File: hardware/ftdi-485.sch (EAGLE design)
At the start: 35 parts, among them IC1 MAX481CSA, J1 NE8FAH, J2 POWER_JACKPTH_LOCK, U1 FT232BL, Y1 6MHz

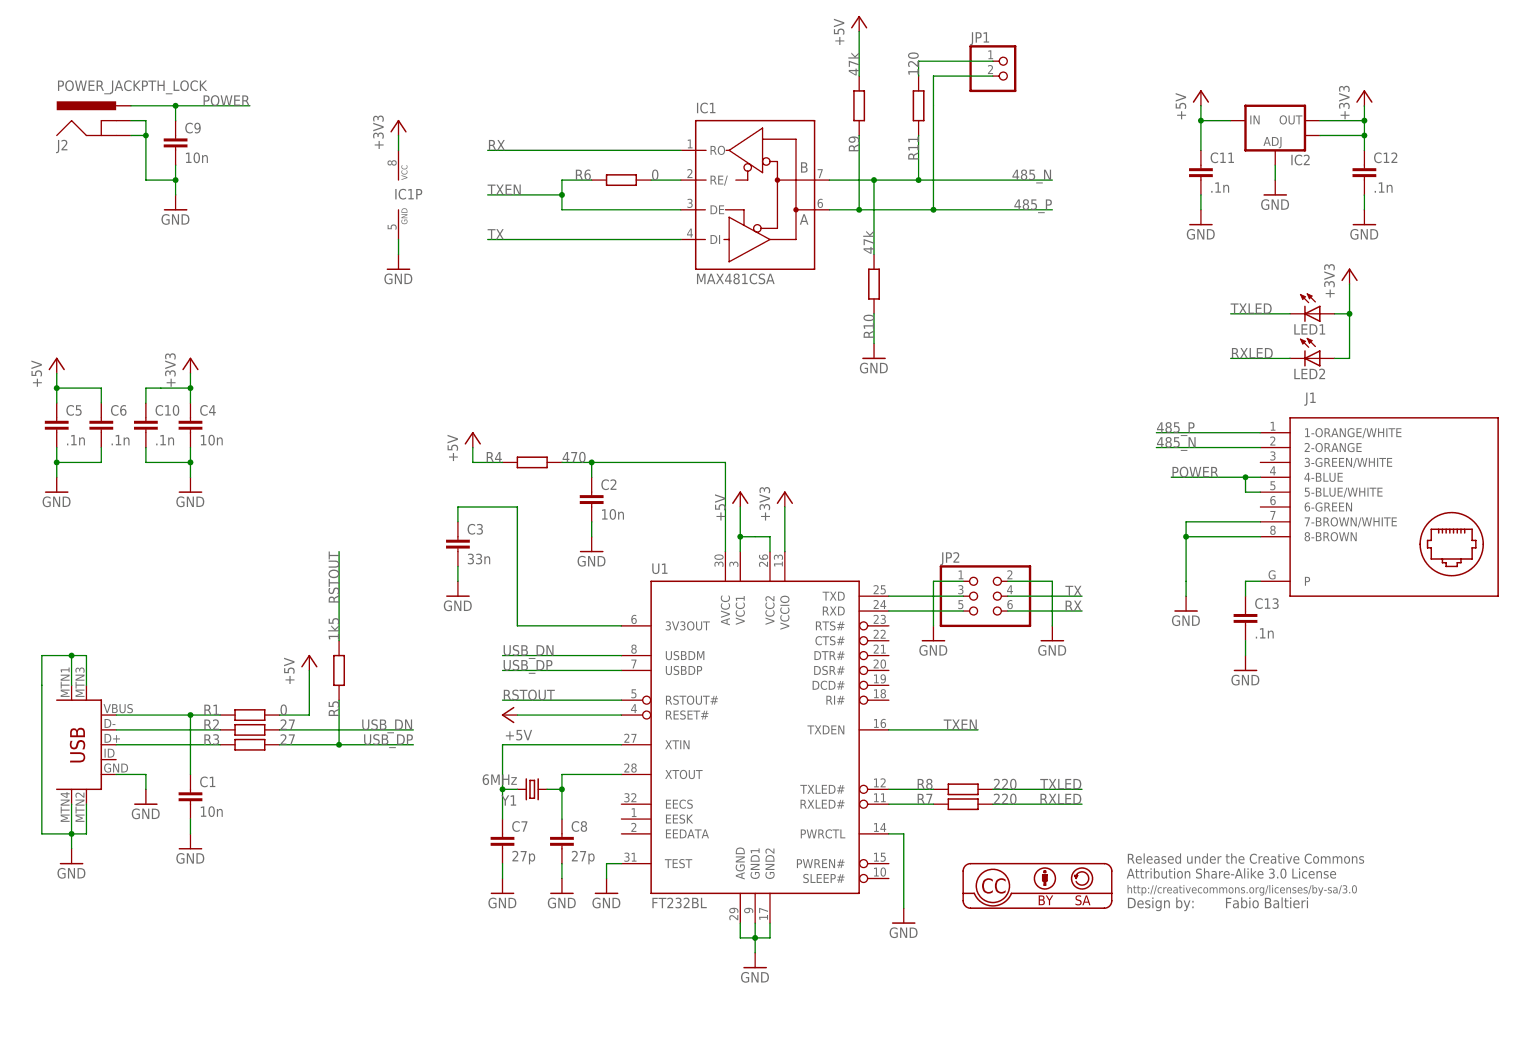
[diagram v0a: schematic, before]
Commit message: hardware: cosmetic changes
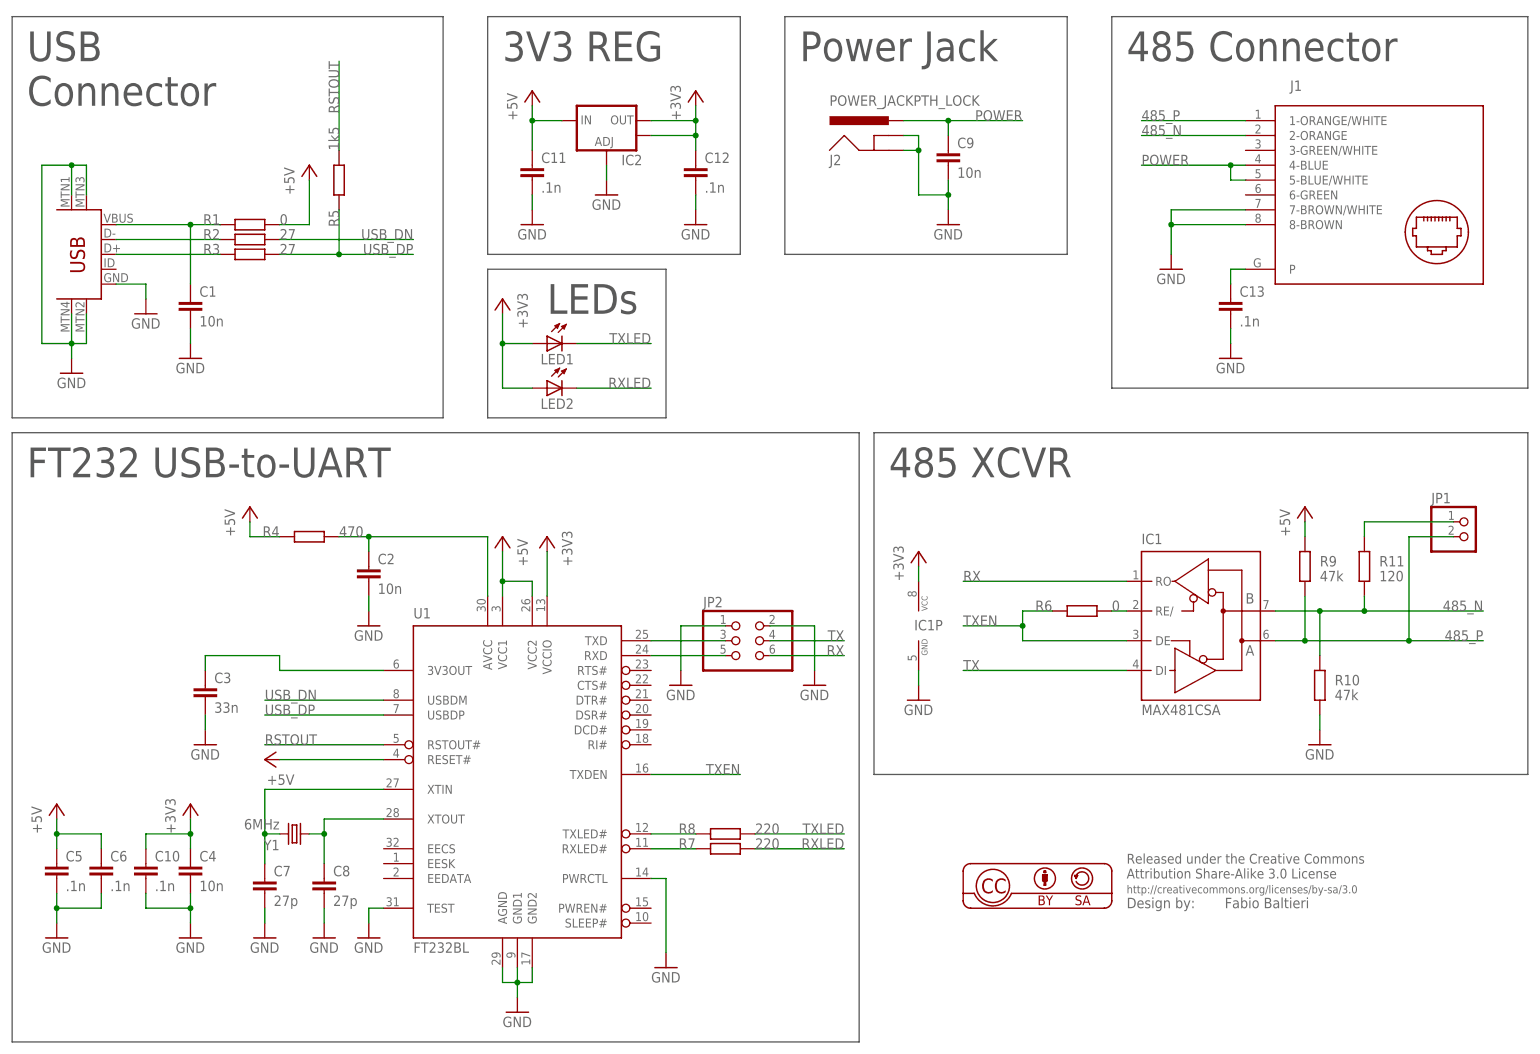
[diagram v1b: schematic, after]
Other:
- note added: "3V3 REG"
- note added: "485 Connector"
- note added: "485 XCVR"
- note added: "Connector"
- note added: "FT232 USB-to-UART"
- note added: "LEDs"
- note added: "Power Jack"
- note added: "USB"
- moved on the sheet: C1, C10, C11, C12, C13, C2, C3, C4, C5, C6, C7, C8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
